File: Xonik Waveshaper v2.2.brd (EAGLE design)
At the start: 55.9 x 21 mm, 78 parts, among them IC1 TL074JT, IC2 TL074JT, IC3 TL074JT, IC4 TL072JT, IC5 4013T, IC6 LM311T, T1 2n3904

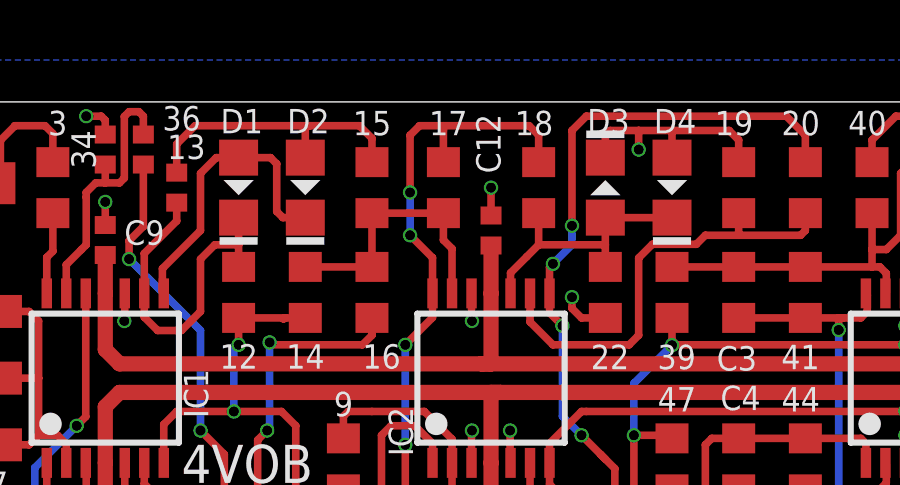
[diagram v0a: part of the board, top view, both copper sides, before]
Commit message: Updated footprints
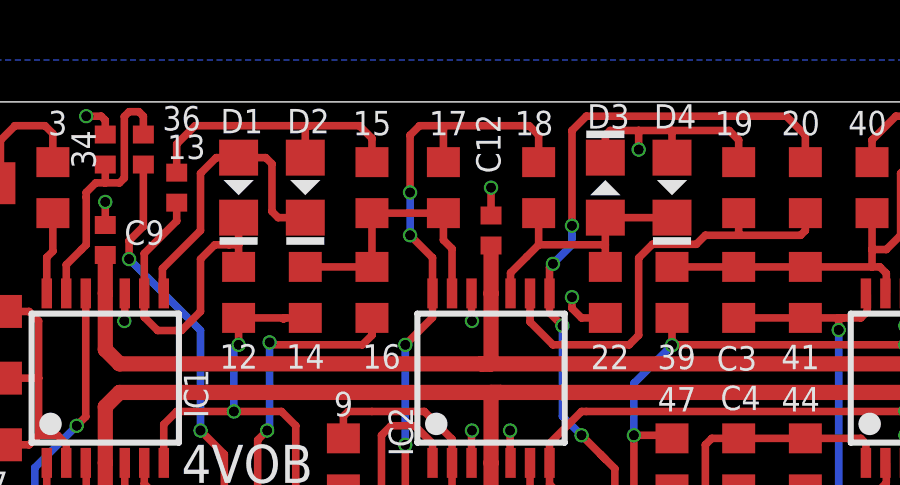
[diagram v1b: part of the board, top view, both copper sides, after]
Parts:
- C1, C14, C2, C3, C4, C5, C6, C7: device joakim:R0603-J -> joakim:C0603-J
- turned D1 to 90 degrees
- turned D2 to 90 degrees
- turned D3 to 270 degrees
- turned D4 to 90 degrees
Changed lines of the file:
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@@
 <attribute name="VALUE" x="21.11375" y="15.24" size="1.27" layer="27" rot="R270"/>
 </element>
-<element name="T1" library="transistor-neu-to92" package="SOT23-BEC" value="2n3904" x="1.905" y="17.145" smashed="yes" rot="R180">
+<element name="T1" library="transistor-neu-to92" library_urn="urn:adsk.eagle:library:397" package="SOT23-BEC" package3d_urn="urn:adsk.eagle:package:28748/2" value="2n3904" x="1.905" y="17.145" smashed="yes" rot="R180">
 <attribute name="NAME" x="1.27" y="19.20875" size="0.8128" layer="25" font="vector"/>
+<attribute name="POPULARITY" value="0" x="1.905" y="17.145" size="1.778" layer="27" rot="R180" display="off"/>
 <attribute name="VALUE" x="3.81" y="20.32" size="1.27" layer="27" rot="R180"/>
 </element>
@@
 <attribute name="VALUE" x="30.00375" y="6.0325" size="1.27" layer="27" rot="R270"/>
 </element>
-<element name="C1" library="joakim" package="R0603-J" value="10pF" x="41.11625" y="5.3975" smashed="yes" rot="R270">
+<element name="C1" library="joakim" package="C0603-J" value="10pF" x="41.11625" y="5.3975" smashed="yes" rot="R270">
 <attribute name="NAME" x="42.00525" y="3.8735" size="0.8128" layer="25" font="vector" rot="R180"/>
 <attribute name="VALUE" x="39.08425" y="6.2865" size="1.27" layer="27" rot="R270"/>
 </element>
-<element name="C2" library="joakim" package="R0603-J" value="10pF" x="39.84625" y="18.0975" smashed="yes" rot="R90">
+<element name="C2" library="joakim" package="C0603-J" value="10pF" x="39.84625" y="18.0975" smashed="yes" rot="R90">
 <attribute name="NAME" x="39.116" y="19.78025" size="0.8128" layer="25" font="vector"/>
 <attribute name="VALUE" x="41.87825" y="17.2085" size="1.27" layer="27" rot="R90"/>
 </element>
-<element name="C3" library="joakim" package="R0603-J" value="30pF" x="27.46375" y="14.605" smashed="yes" rot="R270">
+<element name="C3" library="joakim" package="C0603-J" value="30pF" x="27.46375" y="14.605" smashed="yes" rot="R270">
 <attribute name="NAME" x="26.7335" y="12.0015" size="0.8128" layer="25" font="vector"/>
 <attribute name="VALUE" x="25.43175" y="15.494" size="1.27" layer="27" rot="R270"/>
 </element>
-<element name="C4" library="joakim" package="R0603-J" value="30pF" x="27.46375" y="8.89" smashed="yes" rot="R90">
+<element name="C4" library="joakim" package="C0603-J" value="30pF" x="27.46375" y="8.89" smashed="yes" rot="R90">
 <attribute name="NAME" x="28.194" y="11.4935" size="0.8128" layer="25" font="vector" rot="R180"/>
 <attribute name="VALUE" x="29.49575" y="8.001" size="1.27" layer="27" rot="R90"/>
 </element>
-<element name="C5" library="joakim" package="R0603-J" value="100nF" x="52.86375" y="18.0975" smashed="yes" rot="R270">
+<element name="C5" library="joakim" package="C0603-J" value="100nF" x="52.86375" y="18.0975" smashed="yes" rot="R270">
 <attribute name="NAME" x="53.4035" y="19.78025" size="0.8128" layer="25" font="vector"/>
 <attribute name="VALUE" x="50.83175" y="18.9865" size="1.27" layer="27" rot="R270"/>
 </element>
-<element name="C6" library="joakim" package="R0603-J" value="100nF" x="54.45125" y="5.3975" smashed="yes" rot="R90">
+<element name="C6" library="joakim" package="C0603-J" value="100nF" x="54.45125" y="5.3975" smashed="yes" rot="R90">
 <attribute name="NAME" x="53.721" y="2.95275" size="0.8128" layer="25" font="vector"/>
 <attribute name="VALUE" x="56.48325" y="4.5085" size="1.27" layer="27" rot="R90"/>
 </element>
-<element name="C7" library="joakim" package="R0603-J" value="3pF" x="2.2225" y="9.525" smashed="yes" rot="R180">
+<element name="C7" library="joakim" package="C0603-J" value="3pF" x="2.2225" y="9.525" smashed="yes" rot="R180">
 <attribute name="NAME" x="3.1115" y="8.636" size="0.8128" layer="25" font="vector" rot="R180"/>
 <attribute name="VALUE" x="3.1115" y="11.557" size="1.27" layer="27" rot="R180"/>
@@
 <attribute name="VALUE" x="44.2" y="8.4975" size="1.27" layer="27" rot="R90"/>
 </element>
-<element name="D1" library="joakim" package="D0805-J" value="1N41480805" x="10.795" y="18.0975" smashed="yes" rot="R270">
+<element name="D1" library="joakim" package="D0805-J" value="1N41480805" x="10.795" y="18.0975" smashed="yes" rot="R90">
 <attribute name="NAME" x="10.19175" y="19.90725" size="0.8128" layer="25" font="vector"/>
-<attribute name="VALUE" x="8.509" y="18.8595" size="1.27" layer="27" rot="R270"/>
-</element>
-<element name="D2" library="joakim" package="D0805-J" value="1N41480805" x="13.0175" y="18.0975" smashed="yes" rot="R270">
+<attribute name="VALUE" x="13.081" y="17.3355" size="1.27" layer="27" rot="R90"/>
+</element>
+<element name="D2" library="joakim" package="D0805-J" value="1N41480805" x="13.0175" y="18.0975" smashed="yes" rot="R90">
 <attribute name="NAME" x="12.41425" y="19.90725" size="0.8128" layer="25" font="vector"/>
-<attribute name="VALUE" x="10.7315" y="18.8595" size="1.27" layer="27" rot="R270"/>
-</element>
-<element name="D3" library="joakim" package="D0805-J" value="1N41480805" x="23.01875" y="18.0975" smashed="yes" rot="R90">
-<attribute name="NAME" x="22.4155" y="19.90725" size="0.8128" layer="25" font="vector"/>
-<attribute name="VALUE" x="25.30475" y="17.3355" size="1.27" layer="27" rot="R90"/>
-</element>
-<element name="D4" library="joakim" package="D0805-J" value="1N41480805" x="25.24125" y="18.0975" smashed="yes" rot="R270">
-<attribute name="NAME" x="24.638" y="19.90725" size="0.8128" layer="25" font="vector"/>
-<attribute name="VALUE" x="22.95525" y="18.8595" size="1.27" layer="27" rot="R270"/>
+<attribute name="VALUE" x="15.3035" y="17.3355" size="1.27" layer="27" rot="R90"/>
+</element>
+<element name="D3" library="joakim" package="D0805-J" value="1N41480805" x="23.01875" y="18.0975" smashed="yes" rot="R270">
+<attribute name="NAME" x="22.4155" y="20.066" size="0.8128" layer="25" font="vector"/>
+<attribute name="VALUE" x="20.73275" y="18.8595" size="1.27" layer="27" rot="R270"/>
+</element>
+<element name="D4" library="joakim" package="D0805-J" value="1N41480805" x="25.24125" y="18.0975" smashed="yes" rot="R90">
+<attribute name="NAME" x="24.638" y="20.066" size="0.8128" layer="25" font="vector"/>
+<attribute name="VALUE" x="27.52725" y="17.3355" size="1.27" layer="27" rot="R90"/>
 </element>
 <element name="C16" library="joakim" package="C0402-J" value="1uF" x="33.655" y="6.82625" smashed="yes" rot="R90">
@@
 <attribute name="VALUE" x="48.645" y="8.4975" size="1.27" layer="27" rot="R90"/>
 </element>
-<element name="C14" library="joakim" package="R0603-J" value="820pF" x="46.51375" y="18.0975" smashed="yes" rot="R90">
+<element name="C14" library="joakim" package="C0603-J" value="820pF" x="46.51375" y="18.0975" smashed="yes" rot="R90">
 <attribute name="NAME" x="45.466" y="19.78025" size="0.8128" layer="25" font="vector"/>
 <attribute name="VALUE" x="48.54575" y="17.2085" size="1.27" layer="27" rot="R90"/>
@@
 <wire x1="8.89" y1="13.335" x2="9.525" y2="13.97" width="0.254" layer="1"/>
 <wire x1="9.525" y1="15.71625" x2="10.00125" y2="16.1925" width="0.254" layer="1"/>
-<wire x1="10.00125" y1="16.1925" x2="10.795" y2="16.1925" width="0.254" layer="1"/>
+<wire x1="10.00125" y1="16.1925" x2="10.4775" y2="16.1925" width="0.254" layer="1"/>
+<wire x1="10.4775" y1="16.1925" x2="10.795" y2="16.1925" width="0.254" layer="1"/>
 <wire x1="7.65" y1="13.78125" x2="8.09625" y2="13.335" width="0.254" layer="1"/>
 <wire x1="8.09625" y1="13.335" x2="8.89" y2="13.335" width="0.254" layer="1"/>
@@
 <contactref element="D2" pad="C"/>
 <contactref element="D1" pad="A"/>
-<wire x1="10.795" y1="19.0975" x2="11.85875" y2="19.0975" width="0.254" layer="1"/>
-<wire x1="11.85875" y1="19.0975" x2="12.065" y2="18.89125" width="0.254" layer="1"/>
-<wire x1="12.065" y1="18.89125" x2="12.065" y2="17.30375" width="0.254" layer="1"/>
-<wire x1="12.065" y1="17.30375" x2="12.27125" y2="17.0975" width="0.254" layer="1"/>
-<wire x1="12.27125" y1="17.0975" x2="13.0175" y2="17.0975" width="0.254" layer="1"/>
+<wire x1="10.795" y1="19.0975" x2="11.7" y2="19.0975" width="0.254" layer="1"/>
+<wire x1="11.7" y1="19.0975" x2="11.90625" y2="18.89125" width="0.254" layer="1"/>
+<wire x1="11.90625" y1="18.89125" x2="11.90625" y2="17.30375" width="0.254" layer="1"/>
+<wire x1="11.90625" y1="17.30375" x2="12.1125" y2="17.0975" width="0.254" layer="1"/>
+<wire x1="12.1125" y1="17.0975" x2="13.0175" y2="17.0975" width="0.254" layer="1"/>
 <wire x1="10.795" y1="19.0975" x2="10.04875" y2="19.0975" width="0.254" layer="1"/>
 <wire x1="10.04875" y1="19.0975" x2="9.525" y2="18.57375" width="0.254" layer="1"/>
@@
 <contactref element="15" pad="2"/>
 <contactref element="D2" pad="A"/>
-<wire x1="12.85875" y1="20.16125" x2="13.0175" y2="20.16125" width="0.254" layer="1"/>
 <wire x1="13.0175" y1="20.16125" x2="13.17625" y2="20.16125" width="0.254" layer="1"/>
-<wire x1="12.85875" y1="20.16125" x2="9.3425" y2="20.16125" width="0.254" layer="1"/>
+<wire x1="13.0175" y1="20.16125" x2="9.3425" y2="20.16125" width="0.254" layer="1"/>
 <wire x1="8.73125" y1="18.5975" x2="8.73125" y2="19.55" width="0.254" layer="1"/>
 <wire x1="9.3425" y1="20.16125" x2="8.73125" y2="19.55" width="0.254" layer="1"/>
